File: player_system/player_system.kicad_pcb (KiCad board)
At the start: 2 copper layers, 26 parts, among them U1 STM32G474VEHx

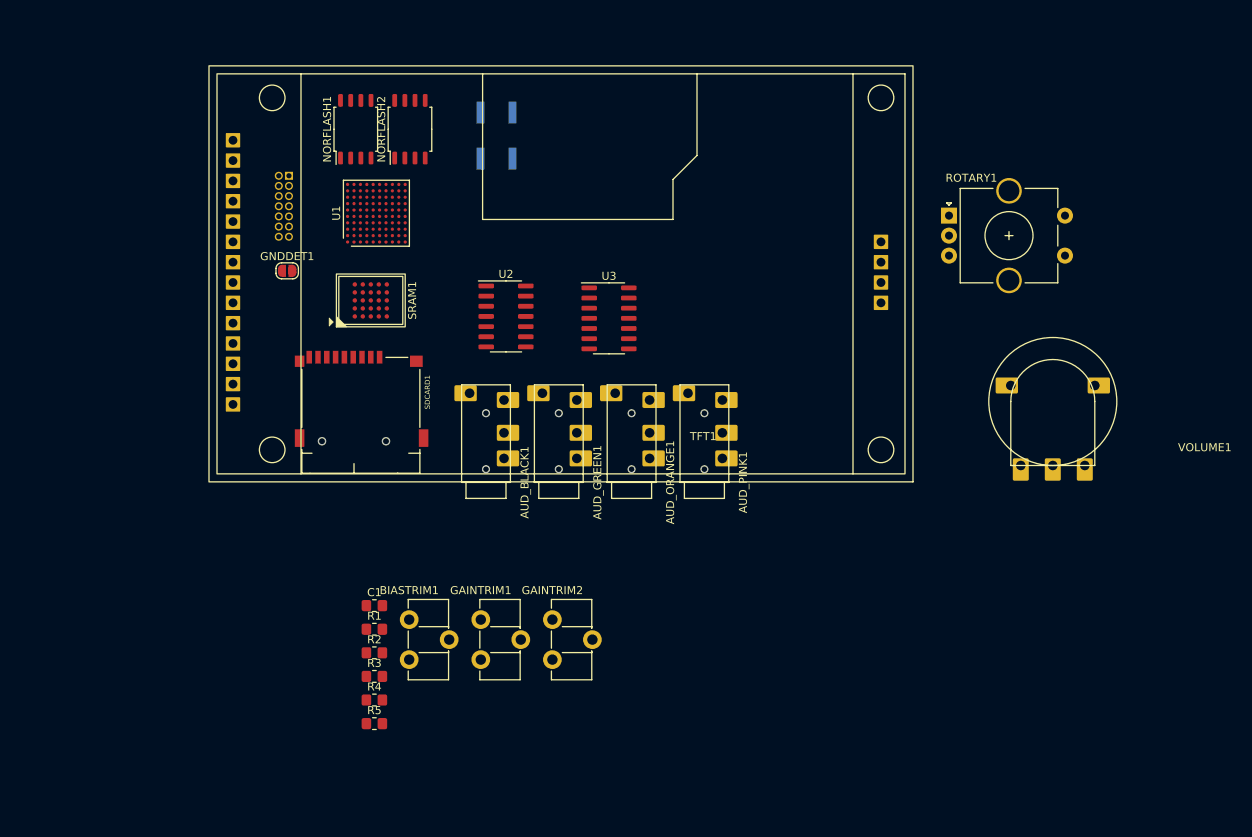
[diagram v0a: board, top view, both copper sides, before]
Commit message: Nearly done with player PCB
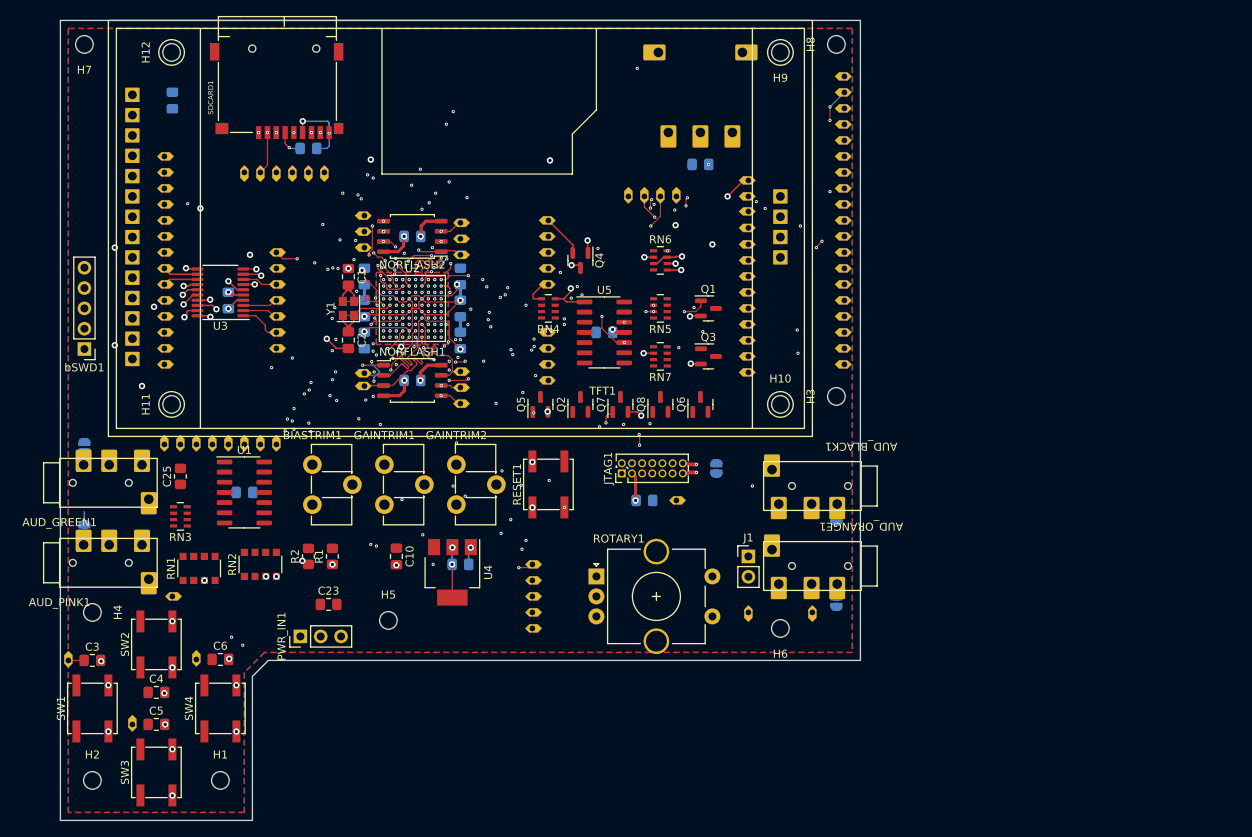
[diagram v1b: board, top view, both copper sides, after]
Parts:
- removed R3, R4, R5: 10k, Resistor_SMD:R_0805_2012Metric_Pad1.20x1.40mm_HandSolder
- removed SRAM1: ~, rtospod_footprints:TFBGA-24-P1.0
- added AUD_GND1: SolderJumper_2_Open, Jumper:SolderJumper-2_P1.3mm_Open_RoundedPad1.0x1.5mm, B.Cu at (90.0, 100.7)
- added AUD_GND2: SolderJumper_2_Open, Jumper:SolderJumper-2_P1.3mm_Open_RoundedPad1.0x1.5mm, B.Cu at (90.0, 90.3)
- added AUD_GND3: SolderJumper_2_Open, Jumper:SolderJumper-2_P1.3mm_Open_RoundedPad1.0x1.5mm, B.Cu at (184.0, 109.7)
- added AUD_GND4: SolderJumper_2_Open, Jumper:SolderJumper-2_P1.3mm_Open_RoundedPad1.0x1.5mm, B.Cu at (184.0, 99.0)
- added C10: 10uf, Capacitor_SMD:C_0805_2012Metric_Pad1.18x1.45mm_HandSolder, F.Cu at (129.0, 104.0)
- added C11: 10uf, Capacitor_SMD:C_0805_2012Metric_Pad1.18x1.45mm_HandSolder, B.Cu at (101.0, 47.0)
- added C12: 10uf, Capacitor_SMD:C_0805_2012Metric_Pad1.18x1.45mm_HandSolder, B.Cu at (131.0, 64.0)
- added C13: 10uf, Capacitor_SMD:C_0805_2012Metric_Pad1.18x1.45mm_HandSolder, B.Cu at (137.0, 77.0)
- added C14: 10uf, Capacitor_SMD:C_0805_2012Metric_Pad1.18x1.45mm_HandSolder, B.Cu at (155.0, 76.0)
- added C15: 10uf, Capacitor_SMD:C_0805_2012Metric_Pad1.18x1.45mm_HandSolder, B.Cu at (160.0, 97.0)
- added C16: 10uf, Capacitor_SMD:C_0805_2012Metric_Pad1.18x1.45mm_HandSolder, B.Cu at (108.0, 72.0)
- added C17: 10uf, Capacitor_SMD:C_0805_2012Metric_Pad1.18x1.45mm_HandSolder, B.Cu at (125.0, 69.0)
- added C18: 10uf, Capacitor_SMD:C_0805_2012Metric_Pad1.18x1.45mm_HandSolder, B.Cu at (137.0, 105.0)
- added C19: 10uf, Capacitor_SMD:C_0805_2012Metric_Pad1.18x1.45mm_HandSolder, B.Cu at (125.0, 77.0)
- added C2: 10pf C0G 2%, Capacitor_SMD:C_0805_2012Metric_Pad1.18x1.45mm_HandSolder, F.Cu at (123.0, 77.0)
- added C20: 10uf, Capacitor_SMD:C_0805_2012Metric_Pad1.18x1.45mm_HandSolder, B.Cu at (125.0, 73.0)
- added C21: 10uf, Capacitor_SMD:C_0805_2012Metric_Pad1.18x1.45mm_HandSolder, B.Cu at (118.0, 53.0)
- added C22: 10uf, Capacitor_SMD:C_0805_2012Metric_Pad1.18x1.45mm_HandSolder, B.Cu at (110.0, 96.0)
- added C23: 10uf, Capacitor_SMD:C_0805_2012Metric_Pad1.18x1.45mm_HandSolder, F.Cu at (120.5, 110.0)
- added C24: 10uf, Capacitor_SMD:C_0805_2012Metric_Pad1.18x1.45mm_HandSolder, B.Cu at (167.0, 55.0)
- added C25: 10u, Resistor_SMD:R_0805_2012Metric_Pad1.20x1.40mm_HandSolder, F.Cu at (102.0, 94.0)
- added C3: 100n, Capacitor_SMD:C_0805_2012Metric_Pad1.18x1.45mm_HandSolder, F.Cu at (91.0, 117.0)
- added C4: 100n, Capacitor_SMD:C_0805_2012Metric_Pad1.18x1.45mm_HandSolder, F.Cu at (99.0, 121.0)
- added C5: 100n, Capacitor_SMD:C_0805_2012Metric_Pad1.18x1.45mm_HandSolder, F.Cu at (99.0, 125.0)
- added C6: 100n, Capacitor_SMD:C_0805_2012Metric_Pad1.18x1.45mm_HandSolder, F.Cu at (107.0, 116.9)
- added C7: 10uf, Capacitor_SMD:C_0805_2012Metric_Pad1.18x1.45mm_HandSolder, B.Cu at (131.0, 82.0)
- added C8: 10uf, Capacitor_SMD:C_0805_2012Metric_Pad1.18x1.45mm_HandSolder, B.Cu at (137.0, 69.0)
- added C9: 10uf, Capacitor_SMD:C_0805_2012Metric_Pad1.18x1.45mm_HandSolder, B.Cu at (137.0, 73.0)
- added H1: MountingHole, MountingHole:MountingHole_2.2mm_M2, F.Cu at (107.0, 132.0)
- added H10: MountingHole, MountingHole:MountingHole_2.2mm_M2, F.Cu at (177.0, 85.0)
- added H11: MountingHole, MountingHole:MountingHole_2.2mm_M2, F.Cu at (100.9, 85.0)
- added H12: MountingHole, MountingHole:MountingHole_2.2mm_M2, F.Cu at (100.9, 41.0)
- added H2: MountingHole, MountingHole:MountingHole_2.2mm_M2, F.Cu at (91.0, 132.0)
- added H3: MountingHole, MountingHole:MountingHole_2.2mm_M2, F.Cu at (184.0, 84.0)
- added H4: MountingHole, MountingHole:MountingHole_2.2mm_M2, F.Cu at (91.0, 111.0)
- added H5: MountingHole, MountingHole:MountingHole_2.2mm_M2, F.Cu at (128.0, 112.0)
- added H6: MountingHole, MountingHole:MountingHole_2.2mm_M2, F.Cu at (177.0, 113.0)
- added H7: MountingHole, MountingHole:MountingHole_2.2mm_M2, F.Cu at (90.0, 40.0)
- added H8: MountingHole, MountingHole:MountingHole_2.2mm_M2, F.Cu at (184.0, 40.0)
- added H9: MountingHole, MountingHole:MountingHole_2.2mm_M2, F.Cu at (177.0, 41.0)
- added J1: ~, Connector_PinHeader_2.54mm:PinHeader_1x02_P2.54mm_Vertical, F.Cu at (173.0, 104.0)
- added NT2: NetTie_2, NetTie:NetTie-2_SMD_Pad0.5mm, F.Cu at (166.0, 92.5)
- added NT3: NetTie_2, NetTie:NetTie-2_SMD_Pad0.5mm, F.Cu at (166.0, 93.5)
- added PWR_IN1: ~, Connector_PinHeader_2.54mm:PinHeader_1x03_P2.54mm_Vertical, F.Cu at (117.0, 114.0)
- added Q1: SI2302, Package_TO_SOT_SMD:SOT-23, F.Cu at (168.0, 73.0)
- added Q2: SI2302, Package_TO_SOT_SMD:SOT-23, F.Cu at (152.0, 85.0)
- added Q3: SI2302, Package_TO_SOT_SMD:SOT-23, F.Cu at (168.0, 79.0)
- added Q4: SI2302, Package_TO_SOT_SMD:SOT-23, F.Cu at (152.0, 67.0)
- added Q5: SI2302, Package_TO_SOT_SMD:SOT-23, F.Cu at (147.0, 85.0)
- added Q6: SI2302, Package_TO_SOT_SMD:SOT-23, F.Cu at (167.0, 85.0)
- added Q7: SI2302, Package_TO_SOT_SMD:SOT-23, F.Cu at (157.0, 85.0)
- added Q8: SI2302, Package_TO_SOT_SMD:SOT-23, F.Cu at (162.0, 85.0)
- added RN1: 1M-1%, Resistor_SMD:R_Array_Convex_4x1206, F.Cu at (104.3, 105.5)
- added RN2: 1M-1%, Resistor_SMD:R_Array_Convex_4x1206, F.Cu at (112.0, 105.0)
- added RN3: 10k, Resistor_SMD:R_Array_Concave_4x0603, F.Cu at (102.0, 99.0)
- added RN4: 10k, Resistor_SMD:R_Array_Concave_4x0603, F.Cu at (148.0, 73.0)
- added RN5: 10k, Resistor_SMD:R_Array_Concave_4x0603, F.Cu at (162.0, 73.0)
- added RN6: 10k, Resistor_SMD:R_Array_Concave_4x0603, F.Cu at (162.0, 67.0)
- added RN7: 10k, Resistor_SMD:R_Array_Concave_4x0603, F.Cu at (162.0, 79.0)
- added SD_DAT1: ., rtospod_footprints:tht_testpt, B.Cu at (110.0, 56.0)
- added SD_DAT2: ., rtospod_footprints:tht_testpt, B.Cu at (120.0, 56.0)
- added SW1: ~, Button_Switch_SMD:SW_SPST_EVPBF, F.Cu at (91.0, 123.0)
- added SW2: ~, Button_Switch_SMD:SW_SPST_EVPBF, F.Cu at (99.0, 115.0)
- added SW3: ~, Button_Switch_SMD:SW_SPST_EVPBF, F.Cu at (99.0, 131.0)
- added SW4: ~, Button_Switch_SMD:SW_SPST_EVPBF, F.Cu at (107.0, 123.0)
- added TP1: ~, rtospod_footprints:tht_testpt, B.Cu at (137.0, 66.3)
- added TP10: ~, rtospod_footprints:tht_testpt, B.Cu at (125.0, 82.7)
- added TP100: ~, rtospod_footprints:tht_testpt, B.Cu at (173.0, 79.0)
- added TP101: ~, rtospod_footprints:tht_testpt, B.Cu at (173.0, 81.0)
- added TP11: ~, rtospod_footprints:tht_testpt, B.Cu at (137.0, 80.9)
- added TP12: ~, rtospod_footprints:tht_testpt, B.Cu at (100.0, 62.0)
- added TP13: ~, rtospod_footprints:tht_testpt, B.Cu at (100.0, 56.0)
- added TP14: ~, rtospod_footprints:tht_testpt, B.Cu at (100.0, 58.0)
- added TP15: ~, rtospod_footprints:tht_testpt, B.Cu at (100.0, 64.0)
- added TP16: ~, rtospod_footprints:tht_testpt, B.Cu at (100.0, 60.0)
- added TP17: ~, rtospod_footprints:tht_testpt, B.Cu at (100.0, 54.0)
- added TP18: ~, rtospod_footprints:tht_testpt, B.Cu at (173.0, 67.0)
- added TP19: ~, rtospod_footprints:tht_testpt, B.Cu at (173.0, 65.0)
- added TP2: ~, rtospod_footprints:tht_testpt, B.Cu at (125.0, 63.4)
- added TP20: ~, rtospod_footprints:tht_testpt, B.Cu at (173.0, 62.9)
- added TP21: ~, rtospod_footprints:tht_testpt, B.Cu at (173.0, 60.9)
- added TP22: ~, rtospod_footprints:tht_testpt, B.Cu at (114.0, 56.0)
- added TP23: ~, rtospod_footprints:tht_testpt, B.Cu at (118.0, 56.0)
- added TP24: ~, rtospod_footprints:tht_testpt, B.Cu at (116.0, 56.0)
- added TP25: ~, rtospod_footprints:tht_testpt, B.Cu at (112.0, 56.0)
- added TP26: ~, rtospod_footprints:tht_testpt, B.Cu at (104.0, 90.0)
- added TP27: ~, rtospod_footprints:tht_testpt, B.Cu at (173.0, 69.0)
- added TP28: ~, rtospod_footprints:tht_testpt, B.Cu at (148.0, 76.0)
- added TP29: ~, rtospod_footprints:tht_testpt, B.Cu at (173.0, 71.0)
- added TP3: ~, rtospod_footprints:tht_testpt, B.Cu at (125.0, 61.4)
- added TP30: ~, rtospod_footprints:tht_testpt, B.Cu at (148.0, 78.0)
- added TP31: ~, rtospod_footprints:tht_testpt, B.Cu at (110.0, 90.0)
- added TP32: ~, rtospod_footprints:tht_testpt, B.Cu at (112.0, 90.0)
- added TP33: ~, rtospod_footprints:tht_testpt, B.Cu at (114.0, 90.0)
- added TP34: ~, rtospod_footprints:tht_testpt, B.Cu at (173.0, 111.0)
- added TP35: ~, rtospod_footprints:tht_testpt, B.Cu at (164.0, 59.0)
- added TP36: ~, rtospod_footprints:tht_testpt, B.Cu at (162.0, 59.0)
- added TP37: ~, rtospod_footprints:tht_testpt, B.Cu at (160.0, 59.0)
- added TP38: ~, rtospod_footprints:tht_testpt, B.Cu at (158.0, 59.0)
- added TP39: ~, rtospod_footprints:tht_testpt, B.Cu at (146.0, 107.0)
- added TP4: ~, rtospod_footprints:tht_testpt, B.Cu at (137.0, 64.3)
- added TP40: ~, rtospod_footprints:tht_testpt, B.Cu at (146.0, 113.0)
- added TP41: ~, rtospod_footprints:tht_testpt, B.Cu at (146.0, 109.0)
- added TP42: ~, rtospod_footprints:tht_testpt, B.Cu at (146.0, 111.0)
- added TP43: ~, rtospod_footprints:tht_testpt, B.Cu at (146.0, 105.0)
- added TP44: ~, rtospod_footprints:tht_testpt, B.Cu at (100.0, 70.0)
- added TP45: ~, rtospod_footprints:tht_testpt, B.Cu at (100.0, 72.0)
- added TP46: ~, rtospod_footprints:tht_testpt, B.Cu at (100.0, 66.0)
- added TP47: ~, rtospod_footprints:tht_testpt, B.Cu at (100.0, 68.0)
- added TP48: ~, rtospod_footprints:tht_testpt, B.Cu at (114.0, 70.0)
- added TP49: ~, rtospod_footprints:tht_testpt, B.Cu at (114.0, 68.0)
- added TP5: ~, rtospod_footprints:tht_testpt, B.Cu at (137.0, 62.3)
- added TP50: ~, rtospod_footprints:tht_testpt, B.Cu at (114.0, 66.0)
- added TP51: ~, rtospod_footprints:tht_testpt, B.Cu at (114.0, 74.0)
- added TP52: ~, rtospod_footprints:tht_testpt, B.Cu at (100.0, 76.0)
- added TP53: ~, rtospod_footprints:tht_testpt, B.Cu at (100.0, 78.0)
- added TP54: ~, rtospod_footprints:tht_testpt, B.Cu at (114.0, 76.0)
- added TP55: ~, rtospod_footprints:tht_testpt, B.Cu at (100.0, 80.0)
- added TP56: ~, rtospod_footprints:tht_testpt, B.Cu at (100.0, 74.0)
- added TP57: ~, rtospod_footprints:tht_testpt, B.Cu at (114.0, 72.0)
- added TP58: ~, rtospod_footprints:tht_testpt, B.Cu at (114.0, 78.0)
- added TP59: ~, rtospod_footprints:tht_testpt, B.Cu at (88.0, 117.0)
- added TP6: ~, rtospod_footprints:tht_testpt, B.Cu at (125.0, 65.4)
- added TP60: ~, rtospod_footprints:tht_testpt, B.Cu at (96.0, 125.0)
- added TP61: ~, rtospod_footprints:tht_testpt, B.Cu at (101.0, 109.0)
- added TP62: ~, rtospod_footprints:tht_testpt, B.Cu at (104.0, 116.9)
- added TP63: ~, rtospod_footprints:tht_testpt, B.Cu at (185.0, 44.0)
- added TP64: ~, rtospod_footprints:tht_testpt, B.Cu at (185.0, 46.0)
- added TP65: ~, rtospod_footprints:tht_testpt, B.Cu at (185.0, 48.0)
- added TP66: ~, rtospod_footprints:tht_testpt, B.Cu at (185.0, 50.0)
- added TP67: ~, rtospod_footprints:tht_testpt, B.Cu at (185.0, 52.0)
- added TP68: ~, rtospod_footprints:tht_testpt, B.Cu at (185.0, 54.0)
- added TP69: ~, rtospod_footprints:tht_testpt, B.Cu at (185.0, 56.0)
- added TP7: ~, rtospod_footprints:tht_testpt, B.Cu at (137.0, 82.9)
- added TP70: ~, rtospod_footprints:tht_testpt, B.Cu at (185.0, 58.0)
- added TP71: ~, rtospod_footprints:tht_testpt, B.Cu at (185.0, 60.0)
- added TP72: ~, rtospod_footprints:tht_testpt, B.Cu at (185.0, 62.0)
- added TP73: ~, rtospod_footprints:tht_testpt, B.Cu at (185.0, 64.0)
- added TP74: ~, rtospod_footprints:tht_testpt, B.Cu at (185.0, 66.0)
- added TP75: ~, rtospod_footprints:tht_testpt, B.Cu at (185.0, 68.0)
- added TP76: ~, rtospod_footprints:tht_testpt, B.Cu at (185.0, 70.0)
- added TP77: ~, rtospod_footprints:tht_testpt, B.Cu at (185.0, 72.0)
- added TP78: ~, rtospod_footprints:tht_testpt, B.Cu at (185.0, 74.0)
- added TP79: ~, rtospod_footprints:tht_testpt, B.Cu at (185.0, 76.0)
- added TP8: ~, rtospod_footprints:tht_testpt, B.Cu at (137.0, 84.9)
- added TP80: ~, rtospod_footprints:tht_testpt, B.Cu at (185.0, 78.0)
- added TP81: ~, rtospod_footprints:tht_testpt, B.Cu at (185.0, 80.0)
- added TP82: ~, rtospod_footprints:tht_testpt, B.Cu at (164.0, 97.0)
- added TP83: ~, rtospod_footprints:tht_testpt, B.Cu at (102.0, 90.0)
- added TP84: ~, rtospod_footprints:tht_testpt, B.Cu at (106.0, 90.0)
- added TP85: ~, rtospod_footprints:tht_testpt, B.Cu at (108.0, 90.0)
- added TP86: ~, rtospod_footprints:tht_testpt, B.Cu at (148.0, 70.0)
- added TP87: ~, rtospod_footprints:tht_testpt, B.Cu at (148.0, 68.0)
- added TP88: ~, rtospod_footprints:tht_testpt, B.Cu at (173.0, 73.0)
- added TP89: ~, rtospod_footprints:tht_testpt, B.Cu at (100.0, 90.0)
- added TP9: ~, rtospod_footprints:tht_testpt, B.Cu at (125.0, 81.1)
- added TP90: ~, rtospod_footprints:tht_testpt, B.Cu at (148.0, 80.0)
- added TP91: ~, rtospod_footprints:tht_testpt, B.Cu at (148.0, 66.0)
- added TP92: ~, rtospod_footprints:tht_testpt, B.Cu at (148.0, 64.0)
- added TP93: ~, rtospod_footprints:tht_testpt, B.Cu at (148.0, 62.0)
- added TP94: ~, rtospod_footprints:tht_testpt, B.Cu at (173.0, 59.0)
- added TP95: ~, rtospod_footprints:tht_testpt, B.Cu at (173.0, 57.0)
- added TP96: ~, rtospod_footprints:tht_testpt, B.Cu at (148.0, 82.0)
- added TP97: ~, rtospod_footprints:tht_testpt, B.Cu at (181.0, 111.0)
- added TP98: ~, rtospod_footprints:tht_testpt, B.Cu at (173.0, 75.0)
- added TP99: ~, rtospod_footprints:tht_testpt, B.Cu at (173.0, 77.0)
- added U4: LDI1117-05H, Package_TO_SOT_SMD:SOT-223-3_TabPin2, F.Cu at (136.0, 106.0)
- added U5: ~, Package_SO:SOIC-14_3.9x8.7mm_P1.27mm, F.Cu at (155.0, 76.0)
- added Y1: 16mhz 10ppm, Crystal:Crystal_SMD_2520-4Pin_2.5x2.0mm, F.Cu at (123.0, 73.0)
- added bSWD1: BRIDGE_SWD, Connector_PinHeader_2.54mm:PinHeader_1x05_P2.54mm_Vertical, F.Cu at (90.0, 78.1)
- C1: value 10u -> 10pf C0G 2%; footprint Resistor_SMD:R_0805_2012Metric_Pad1.20x1.40mm_HandSolder -> Capacitor_SMD:C_0805_2012Metric_Pad1.18x1.45mm_HandSolder
- GNDDET1: moved to B.Cu
- JTAG1, RESET1: moved to F.Cu
- R2: value 10k -> 1k
- ROTARY1: value RotaryEncoder_Switch -> ~
- U1: value STM32G474VEHx -> ~; footprint Package_BGA:TFBGA-100_8x8mm_Layout10x10_P0.8mm -> Package_SO:SOIC-14_3.9x8.7mm_P1.27mm
- U2: value ~ -> STM32G474VEHx; footprint Package_SO:SOIC-14_3.9x8.7mm_P1.27mm -> Package_BGA:TFBGA-100_8x8mm_Layout10x10_P0.8mm
- U3: value ~ -> STM32G030F6Px; footprint Package_SO:SOIC-14_3.9x8.7mm_P1.27mm -> Package_SO:TSSOP-20_4.4x6.5mm_P0.65mm
- VOLUME1: value R_Potentiometer -> 5k; moved to B.Cu
- moved AUD_PINK1 77.9 mm to (86.9, 101.8), turned to 0 degrees
- moved ROTARY1 63.1 mm to (154.0, 106.5)
- moved VOLUME1 60.6 mm to (167.0, 43.0), turned to 180 degrees
- moved AUD_GREEN1 59.4 mm to (86.9, 91.8), turned to 0 degrees
- moved GNDDET1 59.1 mm to (169.0, 93.0), turned to -90 degrees
- moved JTAG1 55.8 mm to (157.2, 93.6), turned to 90 degrees
- moved AUD_BLACK1 50.1 mm to (187.1, 98.2), turned to 180 degrees
- moved U3 48.7 mm to (107.0, 71.0), turned to 180 degrees
- moved RESET1 44.1 mm to (148.0, 95.0), turned to 90 degrees
- moved SDCARD1 43.0 mm to (115.0, 44.0), turned to 0 degrees
- moved C1 41.2 mm to (123.0, 69.0), turned to -90 degrees
- moved U1 38.6 mm to (110.0, 96.0), turned to 0 degrees
- moved AUD_ORANGE1 34.5 mm to (187.1, 108.2), turned to 180 degrees
- moved NORFLASH1 32.2 mm to (131.0, 82.0), turned to 0 degrees
- moved BIASTRIM1 22.8 mm to (118.5, 92.5)
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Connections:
- AUD_BLACK1 pad R1: unconnected-(AUD_BLACK1-PadR1) -> AUD_BLACK_R1_UNBUFFERED_IN
- AUD_BLACK1 pad R2: unconnected-(AUD_BLACK1-PadR2) -> Net-(AUD_GND4-A)
- AUD_BLACK1 pad S: unconnected-(AUD_BLACK1-PadS) -> AUD_BLACK_S_UNBUFFERED_IN
- AUD_BLACK1 pad T: unconnected-(AUD_BLACK1-PadT) -> AUD_BLACK_T_UNBUFFERED_IN
- AUD_ORANGE1 pad R1: unconnected-(AUD_ORANGE1-PadR1) -> /AUD_OUTPUT_AMP2/postamp_audio
- AUD_ORANGE1 pad R2: unconnected-(AUD_ORANGE1-PadR2) -> Net-(AUD_GND3-A)
- AUD_ORANGE1 pad S: unconnected-(AUD_ORANGE1-PadS) -> Net-(J1-Pin_1)
- AUD_ORANGE1 pad T: unconnected-(AUD_ORANGE1-PadT) -> /AUD_OUTPUT_AMP3/postamp_audio
- AUD_PINK1 pad R1: unconnected-(AUD_PINK1-PadR1) -> Net-(RN1A-R1.2)
- AUD_PINK1 pad R2: unconnected-(AUD_PINK1-PadR2) -> Net-(AUD_GND1-A)
- AUD_PINK1 pad S: unconnected-(AUD_PINK1-PadS) -> Net-(RN1D-R4.2)
- AUD_PINK1 pad T: unconnected-(AUD_PINK1-PadT) -> Net-(RN2A-R1.2)
- BIASTRIM1 pad 1: GND -> Net-(U1A-INA-)
- BIASTRIM1 pad 2: Net-(U2A-INA-) -> Net-(U1A-INA-)
- BIASTRIM1 pad 3: Net-(U2A-INA-) -> +3.3V
- C1 pad 1: /GRN_MIC_IN -> GND
- C1 pad 2: Net-(U2A-INA+) -> Net-(U2-PF0)
- GAINTRIM1 pad 1: Net-(U2A-INA-) -> Net-(U1A-INA-)
- GAINTRIM1 pad 2: Net-(U2A-INA-) -> Net-(U1A-INA-)
- GAINTRIM2 pad 3: /mic_aud_conditioning_grn/mic_grn_postamp -> AUD_GRN_MIC_POSTAMP
- JTAG1 pad 3: VDD -> +3.3V
- NORFLASH1 pad 1: unconnected-(NORFLASH1-CE#-Pad1) -> QUADSPI_BK1_NCS
- NORFLASH1 pad 2: unconnected-(NORFLASH1-SO(IO1)-Pad2) -> QUADSPI_BK1_IO1
- NORFLASH1 pad 3: unconnected-(NORFLASH1-WP#(IO2)-Pad3) -> QUADSPI_BK1_IO2
- NORFLASH1 pad 4: unconnected-(NORFLASH1-GND-Pad4) -> GND
- NORFLASH1 pad 5: unconnected-(NORFLASH1-SI(IO0)-Pad5) -> QUADSPI_BK1_IO0
- NORFLASH1 pad 6: unconnected-(NORFLASH1-SCK-Pad6) -> QUADSPI_CLK
- NORFLASH1 pad 7: unconnected-(NORFLASH1-HOLD#(IO3)-Pad7) -> QUADSPI_BK1_IO3
- NORFLASH1 pad 8: unconnected-(NORFLASH1-VCC-Pad8) -> +3.3V
- NORFLASH2 pad 1: unconnected-(NORFLASH2-CE#-Pad1) -> QUADSPI_BK2_NCS
- NORFLASH2 pad 2: unconnected-(NORFLASH2-SO(IO1)-Pad2) -> QUADSPI_BK2_IO1
- NORFLASH2 pad 3: unconnected-(NORFLASH2-WP#(IO2)-Pad3) -> QUADSPI_BK2_IO2
- NORFLASH2 pad 4: unconnected-(NORFLASH2-GND-Pad4) -> GND
- NORFLASH2 pad 5: unconnected-(NORFLASH2-SI(IO0)-Pad5) -> QUADSPI_BK2_IO0
- NORFLASH2 pad 6: unconnected-(NORFLASH2-SCK-Pad6) -> QUADSPI_CLK
- NORFLASH2 pad 7: unconnected-(NORFLASH2-HOLD#(IO3)-Pad7) -> QUADSPI_BK2_IO3
- NORFLASH2 pad 8: unconnected-(NORFLASH2-VCC-Pad8) -> +3.3V
- R1 pad 2: Net-(U2A-INA-) -> Net-(U1A-INA-)
- R2 pad 1: Net-(U2A-INA+) -> GND
- R2 pad 2: +3.3V -> Net-(U1A-INA-)
- ROTARY1 pad A: unconnected-(ROTARY1-PadA) -> ROT_A
- ROTARY1 pad B: unconnected-(ROTARY1-PadB) -> ROT_B
- ROTARY1 pad C: unconnected-(ROTARY1-PadC) -> ROT_C
- ROTARY1 pad S1: unconnected-(ROTARY1-PadS1) -> ROT_S1
- ROTARY1 pad S2: unconnected-(ROTARY1-PadS2) -> ROT_S2
- SDCARD1 pad 1: unconnected-(SDCARD1-DAT2-Pad1) -> Net-(SDCARD1-DAT2)
- SDCARD1 pad 2: unconnected-(SDCARD1-DAT3/CD-Pad2) -> MICRO_SD_CS
- SDCARD1 pad 3: unconnected-(SDCARD1-CMD-Pad3) -> MICRO_SD_MOSI
- SDCARD1 pad 4: unconnected-(SDCARD1-VDD-Pad4) -> +3.3V
- SDCARD1 pad 5: unconnected-(SDCARD1-CLK-Pad5) -> MICRO_SD_SCK
- SDCARD1 pad 6: unconnected-(SDCARD1-VSS-Pad6) -> GND
- SDCARD1 pad 7: unconnected-(SDCARD1-DAT0-Pad7) -> MICRO_SD_MISO
- SDCARD1 pad 8: unconnected-(SDCARD1-DAT1-Pad8) -> Net-(SDCARD1-DAT1)
- SDCARD1 pad 9: unconnected-(SDCARD1-SHIELD-Pad9) -> GND
- TFT1 pad 1: unconnected-(TFT1A-VCC-Pad1) -> +3.3V
- TFT1 pad 10: unconnected-(TFT1C-T_CLK-Pad10) -> BRIDGE_SPI1_SCK
- TFT1 pad 11: unconnected-(TFT1C-T_CS-Pad11) -> BRIDGE_SPI1_NSS
- TFT1 pad 12: unconnected-(TFT1C-T_DIN-Pad12) -> BRIDGE_SPI1_MOSI
- TFT1 pad 13: unconnected-(TFT1C-T_DO-Pad13) -> BRIDGE_SPI1_MISO
- TFT1 pad 14: unconnected-(TFT1C-T_IRQ-Pad14) -> TOUCH_IRQ
- TFT1 pad 15: unconnected-(TFT1B-SD_CS-Pad15) -> SD_CS
- TFT1 pad 16: unconnected-(TFT1B-SD_MOSI-Pad16) -> SD_MOSI
- TFT1 pad 17: unconnected-(TFT1B-SD_MISO-Pad17) -> SD_MISO
- TFT1 pad 18: unconnected-(TFT1B-SD_SCK-Pad18) -> SD_SCK
- TFT1 pad 2: unconnected-(TFT1A-GND-Pad2) -> GND
- TFT1 pad 3: unconnected-(TFT1A-CS-Pad3) -> TFT_SPI_NSS
- TFT1 pad 4: unconnected-(TFT1A-RESET-Pad4) -> TFT_NRST
- TFT1 pad 5: unconnected-(TFT1A-DC-Pad5) -> TFT_SPI_DC
- TFT1 pad 6: unconnected-(TFT1A-MOSI-Pad6) -> TFT_SPI_MOSI
- TFT1 pad 7: unconnected-(TFT1A-SCK-Pad7) -> TFT_SPI_SCK
- TFT1 pad 8: unconnected-(TFT1A-LED_LVL-Pad8) -> TFT_LED_LVL
- TFT1 pad 9: unconnected-(TFT1A-MISO-Pad9) -> TFT_SPI_MISO
- U3 pad 1: unconnected-(U3A-OUTA-Pad1) -> BRIDGE_PB7
- U3 pad 10: unconnected-(U3C-INC+-Pad10) -> BRIDGE_USART_RX
- U3 pad 11: GND -> BRIDGE_SPI1_NSS
- U3 pad 12: unconnected-(U3D-IND+-Pad12) -> BRIDGE_SPI1_SCK
- U3 pad 13: unconnected-(U3D-IND--Pad13) -> BRIDGE_SPI1_MISO
- U3 pad 14: unconnected-(U3D-OUTD-Pad14) -> BRIDGE_SPI1_MOSI
- U3 pad 2: unconnected-(U3A-INA--Pad2) -> BRIDGE_CLK
- U3 pad 3: unconnected-(U3A-INA+-Pad3) -> BRIDGE_PC13
- U3 pad 4: +BATT -> +3.3V
- U3 pad 5: unconnected-(U3B-INB+-Pad5) -> GND
- U3 pad 6: unconnected-(U3B-INB--Pad6) -> BRIDGE_NRST
- U3 pad 7: unconnected-(U3B-OUTB-Pad7) -> TOUCH_IRQ
- U3 pad 8: unconnected-(U3C-OUTA-Pad8) -> BRIDGE_USART_CK
- U3 pad 9: unconnected-(U3C-INC--Pad9) -> BRIDGE_USART_TX
- VOLUME1 pad 1: unconnected-(VOLUME1-Pad1) -> +3.3V
- VOLUME1 pad 2: unconnected-(VOLUME1-Pad2) -> VOLUME_ANALOG_IN
- VOLUME1 pad 3: unconnected-(VOLUME1-Pad3) -> GND
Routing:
- net PB2: track 0.00 -> 125.7 mm, vias 0 -> 9
- net AUD_ORANGE_L_PREAMP_AUDIO: track 0.00 -> 104.7 mm, vias 0 -> 8
- net /GRN_R_AUD_OUT: track 0.00 -> 104.2 mm, vias 0 -> 6
- net PE7: track 0.00 -> 98.3 mm, vias 0 -> 3
- net PA8: track 0.00 -> 97.7 mm, vias 0 -> 5
- net AUD_ORANGE_L_OUTPUT_EN: track 0.00 -> 88.4 mm, vias 0 -> 6
- net PC15: track 0.00 -> 88.4 mm, vias 0 -> 5
- net PA10: track 0.00 -> 86.3 mm, vias 0 -> 3
- net PC13: track 0.00 -> 85.9 mm, vias 0 -> 4
- net PB7: track 0.00 -> 85.4 mm, vias 0 -> 4
- net PE3: track 0.00 -> 84.7 mm, vias 0 -> 3
- net +3.3V: track 0.00 -> 83.1 mm, vias 0 -> 20
- net AUD_GREEN_R_OUTPUT_EN: track 0.00 -> 81.8 mm, vias 0 -> 6
- net PB8: track 0.00 -> 80.4 mm, vias 0 -> 3
- net AUD_GREEN_L_OUTPUT_EN: track 0.00 -> 80.3 mm, vias 0 -> 6
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- added copper zone on F.Cu, net +3.3V
- added copper zone on B.Cu, net GND
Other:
- board outline added: 100 x 100 mm
- copper layers 2 -> 4
